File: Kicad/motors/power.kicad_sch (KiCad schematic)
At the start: 25 parts

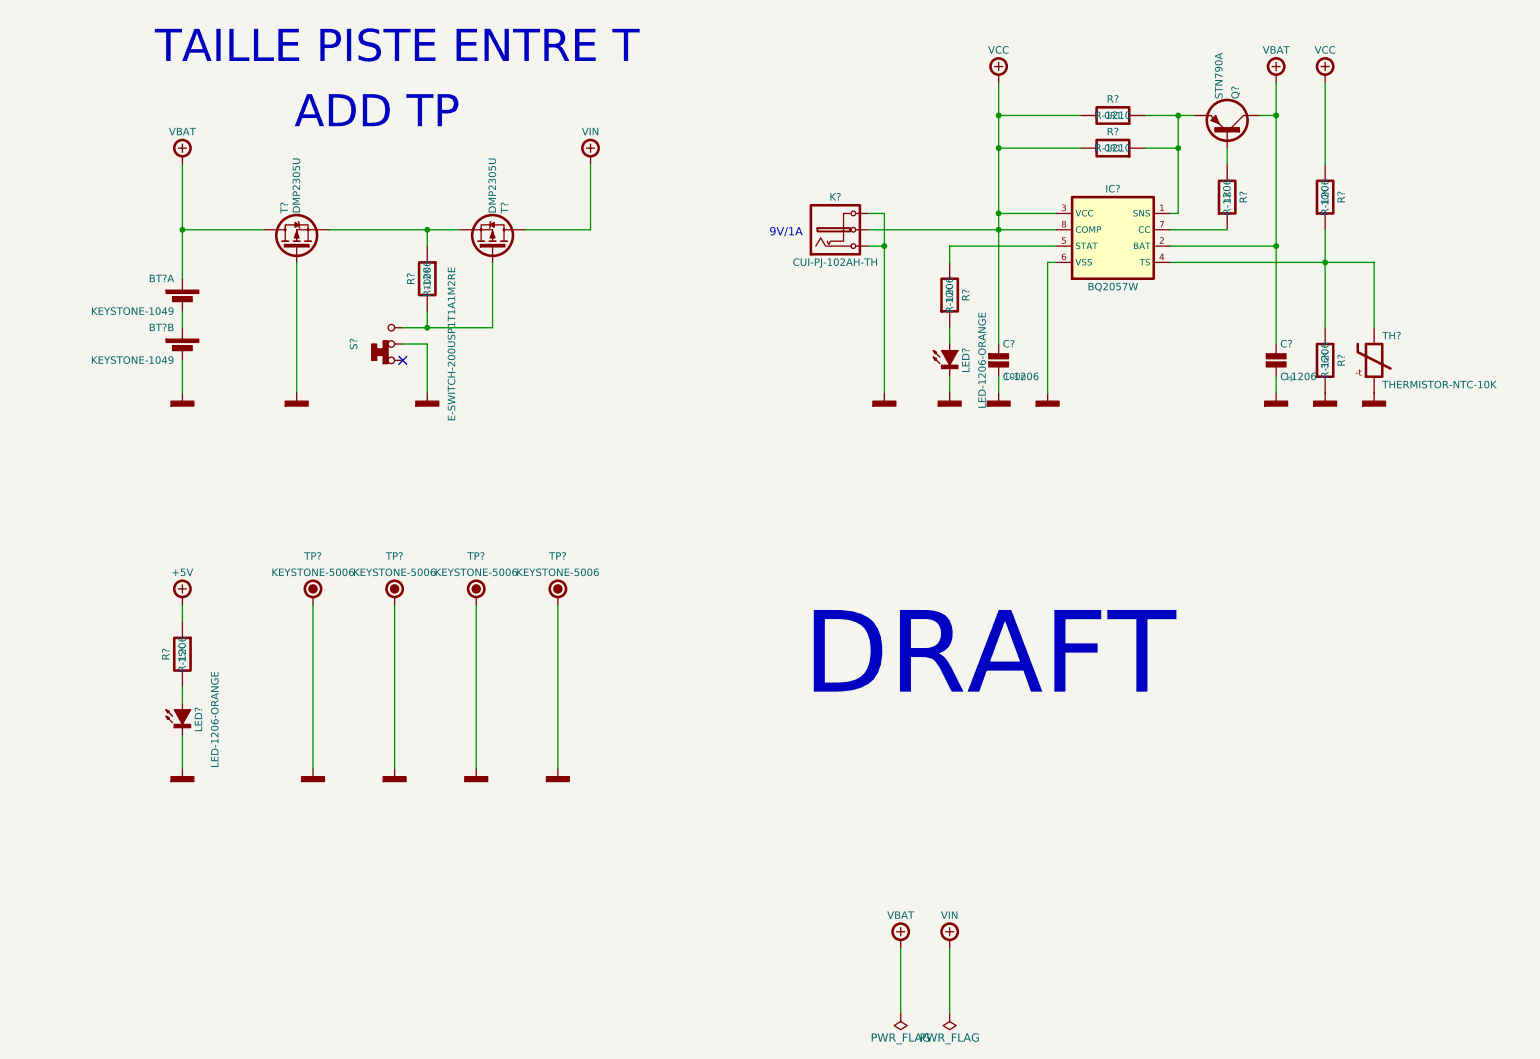
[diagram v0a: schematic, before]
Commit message: Update Motor
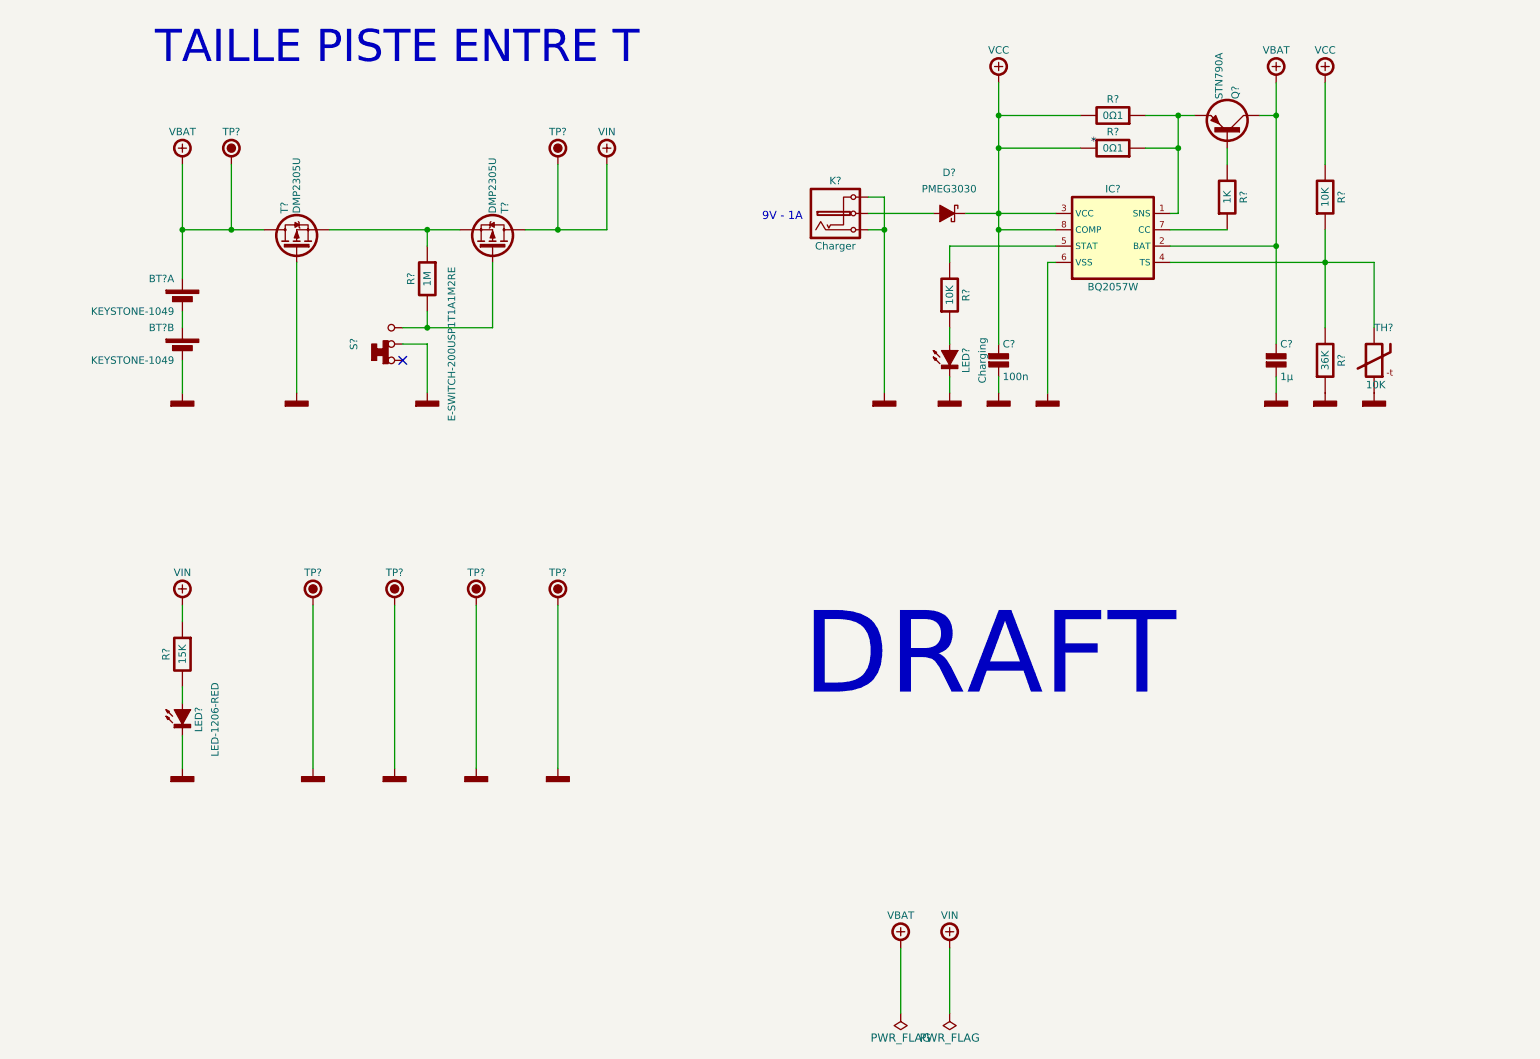
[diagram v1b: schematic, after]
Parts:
- removed TP? (x4): KEYSTONE-5006, tronixio:KEYSTONE-5006, symbol tronixio:KEYSTONE-5006
- added D?: PMEG3030, tronixio:SOD-128, symbol tronixio:PMEG3030
- added TP? (x6): HARWIN-S1751, tronixio:zzzHARWIN-S1751, symbol tronixio:HARWIN-S1751
- C?: value C-1206 -> 100n; Name 100n -> (none)
- C?: value C-1206 -> 1µ; Name 1µ -> (none)
- K?: value CUI-PJ-102AH-TH -> Charger
- LED?: value LED-1206-ORANGE -> Charging; symbol tronixio:LED-1206-ORANGE -> tronixio:LED-1206-RED; MOUSER 604-APT3216LSECKJ4RV -> 604-APT3216LSECKJ3RV
- LED?: value LED-1206-ORANGE -> LED-1206-RED; symbol tronixio:LED-1206-ORANGE -> tronixio:LED-1206-RED; MOUSER 604-APT3216LSECKJ4RV -> 604-APT3216LSECKJ3RV
- R? (x2): value R-1210 -> 0Ω1; Name 0R1 -> (none)
- R?: value R-1206 -> 1K; Name 1K -> (none)
- R?: value R-1206 -> 1M; Name 100K -> (none)
- R? (x2): value R-1206 -> 10K; Name 10K -> (none)
- R?: value R-1206 -> 15K; Name 15K -> (none)
- R?: value R-1206 -> 36K; Name 36K -> (none)
- TH?: value THERMISTOR-NTC-10K -> 10K
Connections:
- net +5V is gone; now on net VIN: R?.2
- net GND: now also TP?.1, TP?.1, TP?.1, TP?.1
- net VBAT: now also TP?.1
- net VCC: now also D?.1 (C); no longer K?.1
- net VIN: now also TP?.1
- new net: D?.2 (A), K?.1
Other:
- note added: "9V - 1A"
- note removed: "9V/1A"
- note removed: "ADD TP"
- moved on the sheet: K?, TH?
